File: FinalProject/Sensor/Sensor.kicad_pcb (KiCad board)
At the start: 2 copper layers, 32.5 x 31 mm, 9 parts, among them J1 Battery, J2 Conn_01x02_Socket, J3 Conn_01x02_Socket, J4 Conn_01x02_Socket, U3 ADS1115IDGS

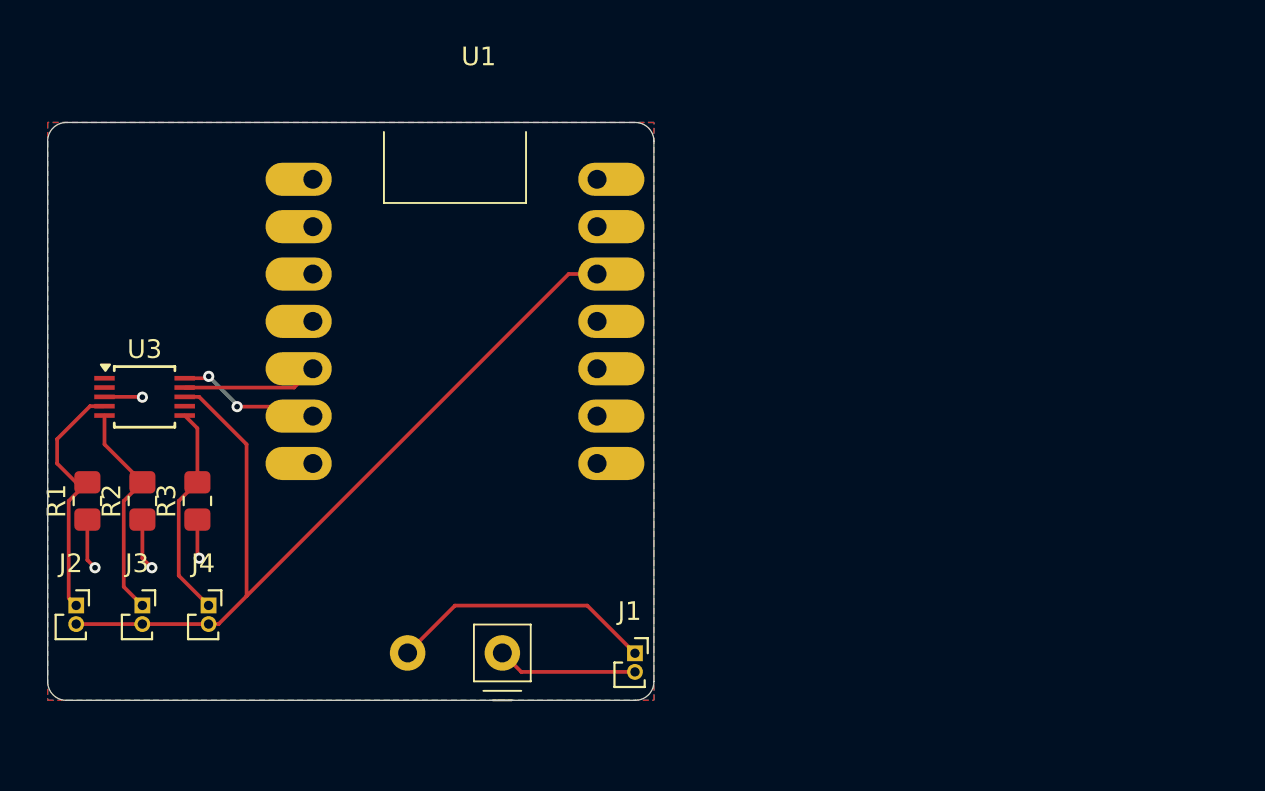
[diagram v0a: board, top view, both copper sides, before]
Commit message: Add pdf
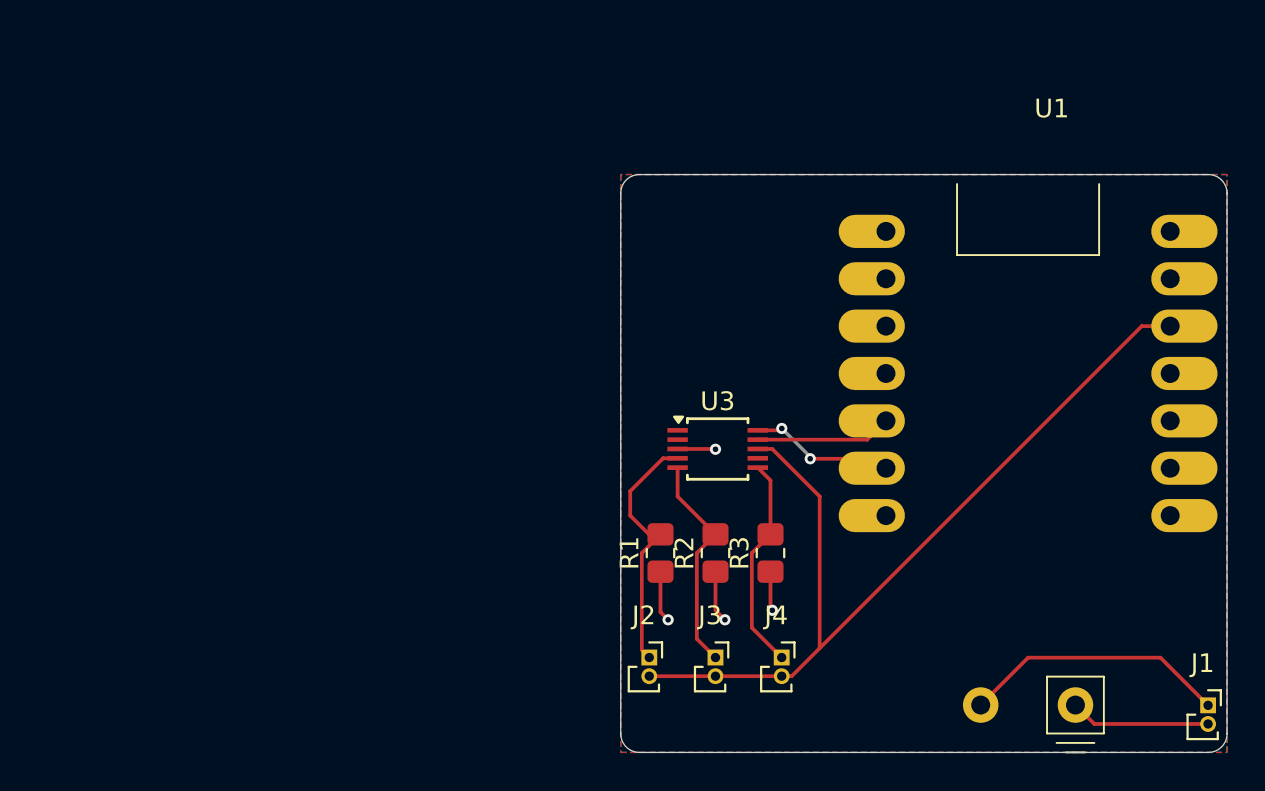
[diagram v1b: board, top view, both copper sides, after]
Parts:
- moved J2 30.9 mm to (141.5, 105.4)
- moved J4 30.9 mm to (148.6, 105.4)
- moved R1 30.9 mm to (142.1, 99.8)
- moved R3 30.9 mm to (148.0, 99.8)
- moved U1 30.9 mm to (161.8, 90.2)
- moved J3 30.9 mm to (145.0, 105.4)
- moved R2 30.9 mm to (145.0, 99.8)
- moved J1 30.9 mm to (171.4, 108.0)
- moved U3 30.9 mm to (145.2, 94.2)
